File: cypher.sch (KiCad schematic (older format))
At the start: 25 parts, among them J3 Breakout, Q1 BC850, Q2 MMBT3904, SW1 SW_Push, U1 STM32F072CBTx, U2 PRTR5V0U2X, U3 LD3985G33R_TSOT23

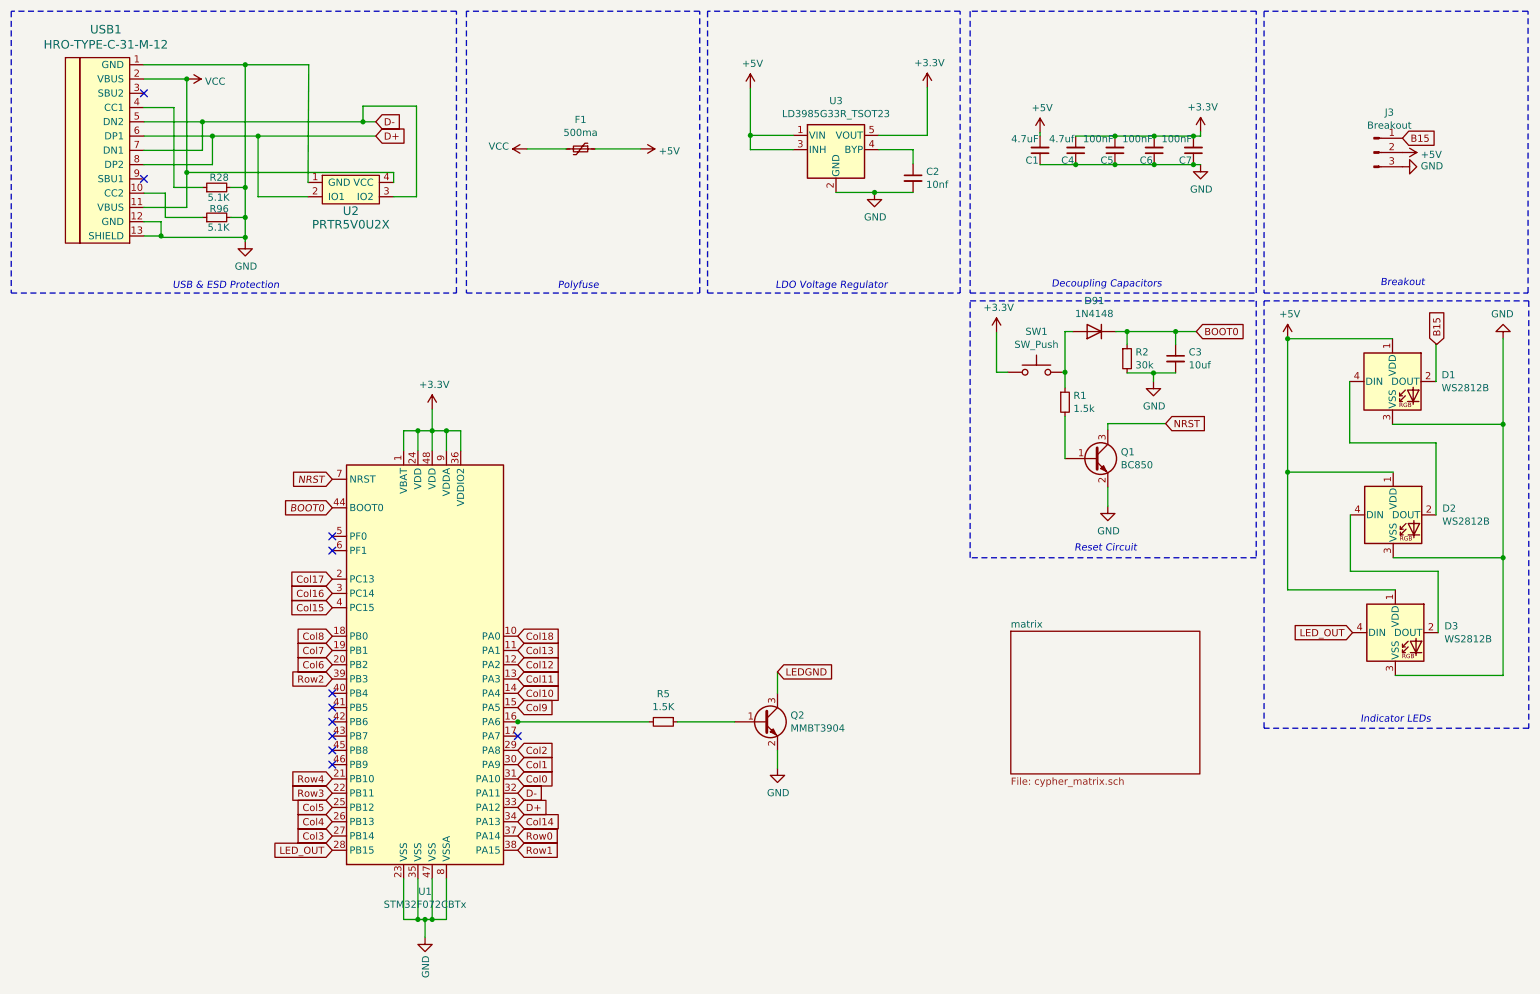
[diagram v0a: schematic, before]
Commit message: updated rev6
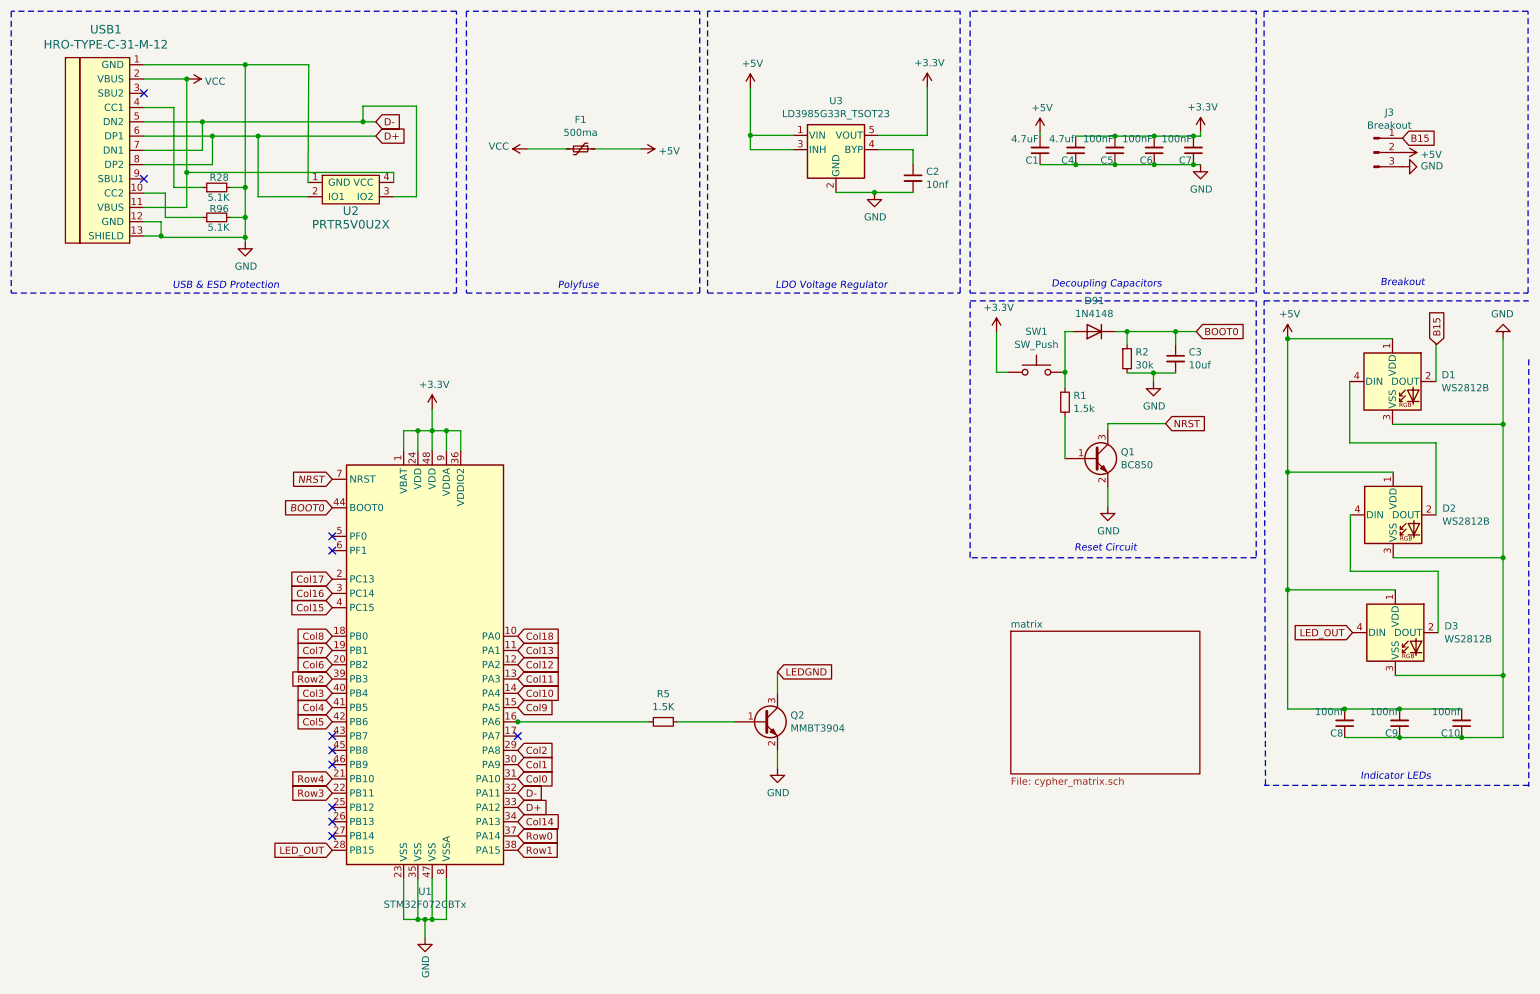
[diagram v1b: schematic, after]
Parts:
- added C10, C8, C9: 100nf, Capacitor_SMD:C_0603_1608Metric, symbol Device:C_Small
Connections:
- net +5V: now also C10.2, C8.2, C9.2
- net Col3: now also U1.40 (PB4); no longer U1.27 (PB14)
- net Col4: now also U1.41 (PB5); no longer U1.26 (PB13)
- net Col5: now also U1.42 (PB6); no longer U1.25 (PB12)
- net GND: now also C10.1, C8.1, C9.1
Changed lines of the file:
@@
 Text GLabel 4080 5755 2    50   Input ~ 0
 Col2
-Text GLabel 2780 6355 0    50   Input ~ 0
+Text GLabel 2780 5355 0    50   Input ~ 0
 Col3
-Text GLabel 2780 6255 0    50   Input ~ 0
+Text GLabel 2780 5455 0    50   Input ~ 0
 Col4
-Text GLabel 2780 6155 0    50   Input ~ 0
+Text GLabel 2780 5555 0    50   Input ~ 0
 Col5
 Text GLabel 2780 5155 0    50   Input ~ 0
@@
 	9310 2605 11165 2605
 Wire Notes Line
-	11165 2605 11165 5600
-Wire Notes Line
-	11165 5600 9310 5600
-Wire Notes Line
-	9310 5600 9310 2605
+	11165 3015 11165 6010
+Wire Notes Line
+	11165 6000 9310 6000
+Wire Notes Line
+	9320 6000 9310 2605
 Text Notes 10125 2510 0    50   Italic 0
 Breakout\n
-Text Notes 9985 5570 0    50   Italic 0
+Text Notes 9985 5970 0    50   Italic 0
 Indicator LEDs\n
 Wire Notes Line
@@
 Wire Wire Line
 	10230 4630 9475 4630
-Wire Wire Line
-	9475 4630 9475 3805
 Connection ~ 9475 3805
 Wire Wire Line
@@
 $EndComp
 NoConn ~ 2780 5855
-NoConn ~ 2780 5355
-NoConn ~ 2780 5455
 NoConn ~ 2780 5755
 NoConn ~ 4080 5655
 NoConn ~ 2780 5655
-NoConn ~ 2780 5555
 Text GLabel 9930 4930 0    50   Input ~ 0
 LED_OUT
@@
 	0    1    1    0
 $EndComp
+NoConn ~ 2780 6155
+NoConn ~ 2780 6255
+NoConn ~ 2780 6355
+$Comp
+L Device:C_Small C8
+U 1 1 5EDBC859
+P 9875 5565
+F 0 "C8" H 9885 5635 50  0000 L CNN
+F 1 "100nf" H 9885 5485 50  0000 L CNN
+F 2 "Capacitor_SMD:C_0603_1608Metric" H 9875 5565 50  0001 C CNN
+F 3 "~" H 9875 5565 50  0001 C CNN
+	1    9875 5565
+	-1   0    0    1
+$EndComp
+$Comp
+L Device:C_Small C9
+U 1 1 5EDBDAFF
+P 10260 5565
+F 0 "C9" H 10270 5635 50  0000 L CNN
+F 1 "100nf" H 10270 5485 50  0000 L CNN
+F 2 "Capacitor_SMD:C_0603_1608Metric" H 10260 5565 50  0001 C CNN
+F 3 "~" H 10260 5565 50  0001 C CNN
+	1    10260 5565
+	-1   0    0    1
+$EndComp
+$Comp
+L Device:C_Small C10
+U 1 1 5EDBE225
+P 10695 5565
+F 0 "C10" H 10705 5635 50  0000 L CNN
+F 1 "100nf" H 10705 5485 50  0000 L CNN
+F 2 "Capacitor_SMD:C_0603_1608Metric" H 10695 5565 50  0001 C CNN
+F 3 "~" H 10695 5565 50  0001 C CNN
+	1    10695 5565
+	-1   0    0    1
+$EndComp
+Connection ~ 10985 5230
+Wire Wire Line
+	10985 5230 10985 5665
+Wire Wire Line
+	10985 5665 10695 5665
+Connection ~ 10260 5665
+Wire Wire Line
+	10260 5665 9875 5665
+Connection ~ 10695 5665
+Wire Wire Line
+	10695 5665 10260 5665
+Wire Wire Line
+	10695 5465 10260 5465
+Wire Wire Line
+	9475 3805 9475 4630
+Connection ~ 9875 5465
+Wire Wire Line
+	9875 5465 9475 5465
+Connection ~ 10260 5465
+Wire Wire Line
+	10260 5465 9875 5465
+Connection ~ 9475 4630
+Wire Wire Line
+	9475 4630 9475 5465
 $EndSCHEMATC
